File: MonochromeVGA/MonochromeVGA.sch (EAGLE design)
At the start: 12 parts

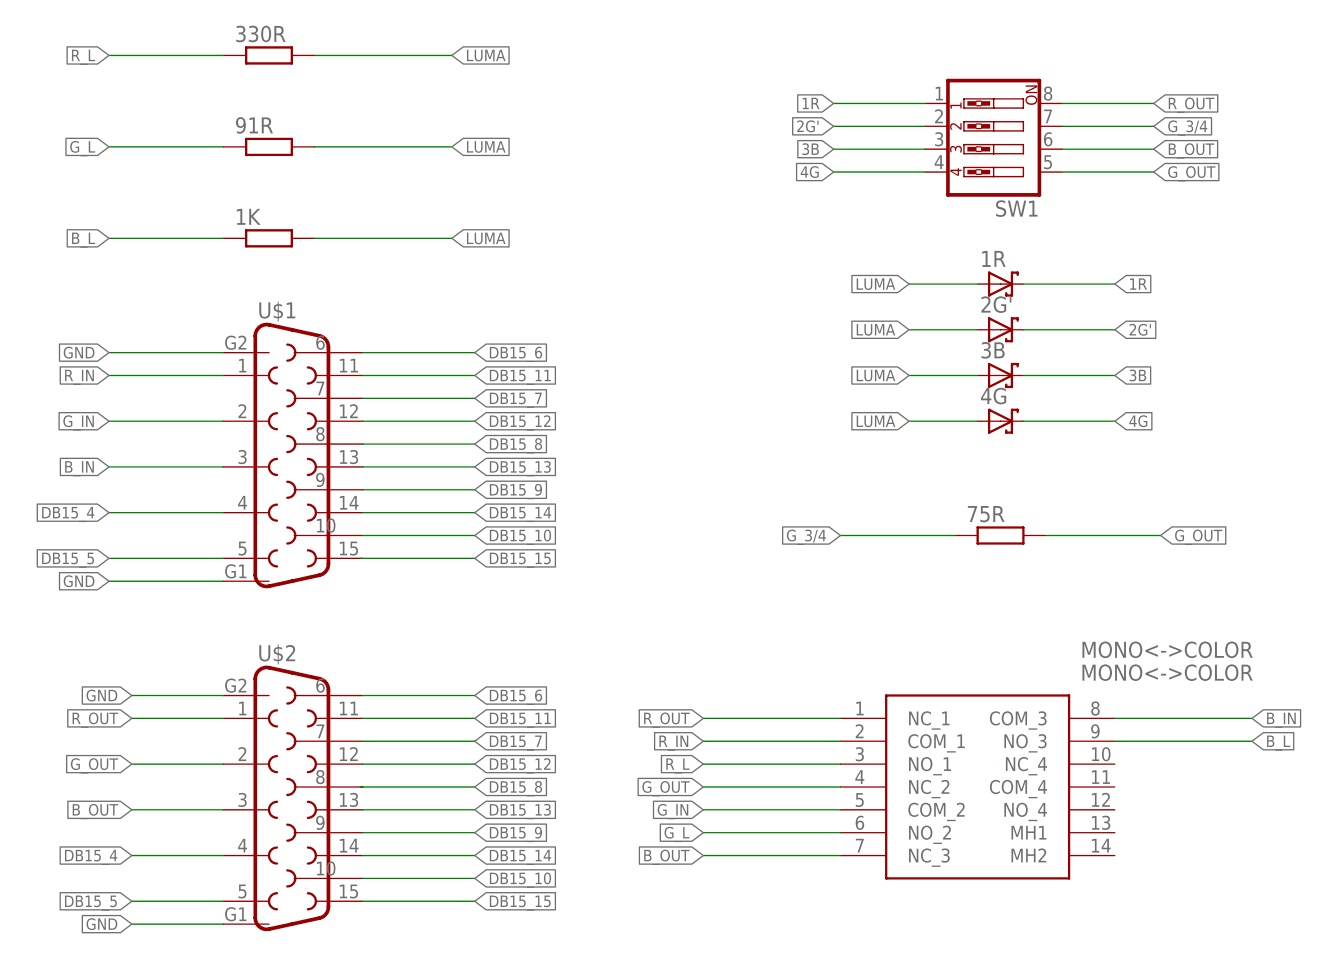
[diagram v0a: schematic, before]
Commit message: Add files via upload
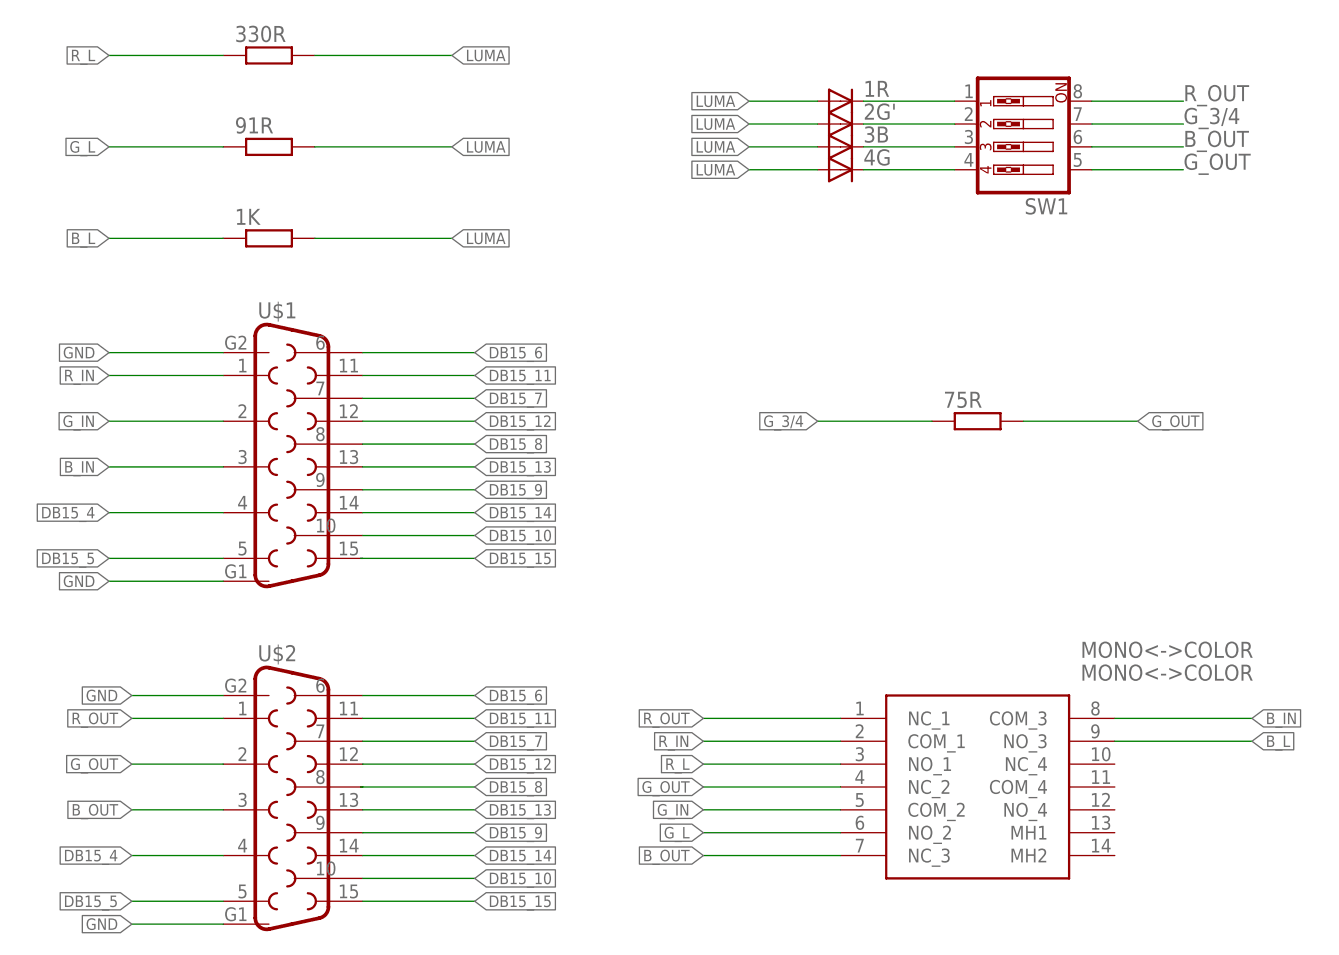
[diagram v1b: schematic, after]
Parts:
- 1R, 2G', 3B, 4G: device diode:SCHOTTKY-DIODEDO35-7 -> diode:DIODE-D-5
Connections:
- net 1R renamed N$6
- net 2G' renamed N$3
- net 3B renamed N$4
- net 4G renamed N$5
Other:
- moved on the sheet: 75R, SW1
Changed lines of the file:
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@@
 <part name="75R" library="resistor" deviceset="R-EU_" device="0204/5"/>
 <part name="MONO&lt;-&gt;COLOR" library="EG4208A" deviceset="EG4208A" device="" value="MONO&lt;-&gt;COLOR"/>
-<part name="2G'" library="diode" deviceset="SCHOTTKY-DIODE" device="DO35-7"/>
-<part name="3B" library="diode" deviceset="SCHOTTKY-DIODE" device="DO35-7"/>
-<part name="4G" library="diode" deviceset="SCHOTTKY-DIODE" device="DO35-7"/>
-<part name="1R" library="diode" deviceset="SCHOTTKY-DIODE" device="DO35-7"/>
+<part name="2G'" library="diode" deviceset="DIODE-" device="D-5"/>
+<part name="3B" library="diode" deviceset="DIODE-" device="D-5"/>
+<part name="4G" library="diode" deviceset="DIODE-" device="D-5"/>
+<part name="1R" library="diode" deviceset="DIODE-" device="D-5"/>
 </parts>
 <sheets>
@@
 </plain>
 <instances>
-<instance part="SW1" gate="A" x="93.218" y="86.106" rot="R180"/>
+<instance part="SW1" gate="A" x="96.52" y="86.36" rot="R180"/>
 <instance part="U$1" gate="G$1" x="15.24" y="53.34"/>
 <instance part="U$2" gate="G$1" x="15.24" y="15.24"/>
@@
 <instance part="91R" gate="G$1" x="12.7" y="86.36"/>
 <instance part="1K" gate="G$1" x="12.7" y="76.2"/>
-<instance part="75R" gate="G$1" x="93.98" y="43.18"/>
+<instance part="75R" gate="G$1" x="91.44" y="55.88"/>
 <instance part="MONO&lt;-&gt;COLOR" gate="G$1" x="76.2" y="22.86"/>
-<instance part="2G'" gate="G$1" x="93.98" y="66.04"/>
-<instance part="3B" gate="G$1" x="93.98" y="60.96"/>
-<instance part="4G" gate="G$1" x="93.98" y="55.88"/>
-<instance part="1R" gate="G$1" x="93.98" y="71.12"/>
+<instance part="2G'" gate="G$1" x="76.2" y="88.9"/>
+<instance part="3B" gate="G$1" x="76.2" y="86.36"/>
+<instance part="4G" gate="G$1" x="76.2" y="83.82"/>
+<instance part="1R" gate="G$1" x="76.2" y="91.44"/>
 </instances>
 <busses>
@@
 <segment>
 <pinref part="2G'" gate="G$1" pin="A"/>
-<wire x1="91.44" y1="66.04" x2="83.82" y2="66.04" width="0.1524" layer="91"/>
-<label x="83.82" y="66.04" size="1.27" layer="95" rot="R180" xref="yes"/>
+<wire x1="73.66" y1="88.9" x2="66.04" y2="88.9" width="0.1524" layer="91"/>
+<label x="66.04" y="88.9" size="1.27" layer="95" rot="R180" xref="yes"/>
 </segment>
 <segment>
 <pinref part="3B" gate="G$1" pin="A"/>
-<wire x1="91.44" y1="60.96" x2="83.82" y2="60.96" width="0.1524" layer="91"/>
-<label x="83.82" y="60.96" size="1.27" layer="95" rot="R180" xref="yes"/>
+<wire x1="73.66" y1="86.36" x2="66.04" y2="86.36" width="0.1524" layer="91"/>
+<label x="66.04" y="86.36" size="1.27" layer="95" rot="R180" xref="yes"/>
 </segment>
 <segment>
 <pinref part="4G" gate="G$1" pin="A"/>
-<wire x1="91.44" y1="55.88" x2="83.82" y2="55.88" width="0.1524" layer="91"/>
-<label x="83.82" y="55.88" size="1.27" layer="95" rot="R180" xref="yes"/>
+<wire x1="73.66" y1="83.82" x2="66.04" y2="83.82" width="0.1524" layer="91"/>
+<label x="66.04" y="83.82" size="1.27" layer="95" rot="R180" xref="yes"/>
 </segment>
 <segment>
 <pinref part="1R" gate="G$1" pin="A"/>
-<wire x1="91.44" y1="71.12" x2="83.82" y2="71.12" width="0.1524" layer="91"/>
-<label x="83.82" y="71.12" size="1.27" layer="95" rot="R180" xref="yes"/>
+<wire x1="73.66" y1="91.44" x2="66.04" y2="91.44" width="0.1524" layer="91"/>
+<label x="66.04" y="91.44" size="1.27" layer="95" rot="R180" xref="yes"/>
 </segment>
 </net>
@@
 <segment>
 <pinref part="SW1" gate="A" pin="8"/>
-<wire x1="100.838" y1="91.186" x2="110.998" y2="91.186" width="0.1524" layer="91"/>
-<label x="110.998" y="91.186" size="1.27" layer="95" xref="yes"/>
+<wire x1="104.14" y1="91.44" x2="114.3" y2="91.44" width="0.1524" layer="91"/>
+<label x="114.3" y="91.44" size="1.778" layer="95"/>
 </segment>
 <segment>
@@
 <segment>
 <pinref part="SW1" gate="A" pin="5"/>
-<wire x1="100.838" y1="83.566" x2="110.998" y2="83.566" width="0.1524" layer="91"/>
-<label x="110.998" y="83.566" size="1.27" layer="95" xref="yes"/>
+<wire x1="104.14" y1="83.82" x2="114.3" y2="83.82" width="0.1524" layer="91"/>
+<label x="114.3" y="83.82" size="1.778" layer="95"/>
 </segment>
 <segment>
@@
 <segment>
 <pinref part="75R" gate="G$1" pin="2"/>
-<wire x1="99.06" y1="43.18" x2="111.76" y2="43.18" width="0.1524" layer="91"/>
-<label x="111.76" y="43.18" size="1.27" layer="95" xref="yes"/>
+<wire x1="96.52" y1="55.88" x2="109.22" y2="55.88" width="0.1524" layer="91"/>
+<label x="109.22" y="55.88" size="1.27" layer="95" xref="yes"/>
 </segment>
 </net>
@@
 <segment>
 <pinref part="SW1" gate="A" pin="6"/>
-<wire x1="100.838" y1="86.106" x2="110.998" y2="86.106" width="0.1524" layer="91"/>
-<label x="110.998" y="86.106" size="1.27" layer="95" xref="yes"/>
+<wire x1="104.14" y1="86.36" x2="114.3" y2="86.36" width="0.1524" layer="91"/>
+<label x="114.3" y="86.36" size="1.778" layer="95"/>
 </segment>
 <segment>
@@
 <segment>
 <pinref part="SW1" gate="A" pin="7"/>
-<wire x1="100.838" y1="88.646" x2="110.998" y2="88.646" width="0.1524" layer="91"/>
-<label x="110.998" y="88.646" size="1.27" layer="95" xref="yes"/>
+<wire x1="104.14" y1="88.9" x2="114.3" y2="88.9" width="0.1524" layer="91"/>
+<label x="114.3" y="88.9" size="1.778" layer="95"/>
 </segment>
 <segment>
 <pinref part="75R" gate="G$1" pin="1"/>
-<wire x1="88.9" y1="43.18" x2="76.2" y2="43.18" width="0.1524" layer="91"/>
-<label x="76.2" y="43.18" size="1.27" layer="95" rot="R180" xref="yes"/>
+<wire x1="86.36" y1="55.88" x2="73.66" y2="55.88" width="0.1524" layer="91"/>
+<label x="73.66" y="55.88" size="1.27" layer="95" rot="R180" xref="yes"/>
 </segment>
 </net>
@@
 </segment>
 </net>
-<net name="1R" class="0">
+<net name="N$3" class="0">
+<segment>
+<pinref part="2G'" gate="G$1" pin="C"/>
+<pinref part="SW1" gate="A" pin="2"/>
+<wire x1="78.74" y1="88.9" x2="88.9" y2="88.9" width="0.1524" layer="91"/>
+</segment>
+</net>
+<net name="N$4" class="0">
+<segment>
+<pinref part="3B" gate="G$1" pin="C"/>
+<pinref part="SW1" gate="A" pin="3"/>
+<wire x1="78.74" y1="86.36" x2="88.9" y2="86.36" width="0.1524" layer="91"/>
+</segment>
+</net>
+<net name="N$5" class="0">
+<segment>
+<pinref part="4G" gate="G$1" pin="C"/>
+<pinref part="SW1" gate="A" pin="4"/>
+<wire x1="78.74" y1="83.82" x2="88.9" y2="83.82" width="0.1524" layer="91"/>
+</segment>
+</net>
+<net name="N$6" class="0">
 <segment>
 <pinref part="1R" gate="G$1" pin="C"/>
-<wire x1="96.52" y1="71.12" x2="106.68" y2="71.12" width="0.1524" layer="91"/>
-<label x="106.68" y="71.12" size="1.27" layer="95" xref="yes"/>
-</segment>
-<segment>
 <pinref part="SW1" gate="A" pin="1"/>
-<wire x1="85.598" y1="91.186" x2="75.438" y2="91.186" width="0.1524" layer="91"/>
-<label x="75.438" y="91.186" size="1.27" layer="95" rot="R180" xref="yes"/>
-</segment>
-</net>
-<net name="2G'" class="0">
-<segment>
-<pinref part="2G'" gate="G$1" pin="C"/>
-<wire x1="96.52" y1="66.04" x2="106.68" y2="66.04" width="0.1524" layer="91"/>
-<label x="106.68" y="66.04" size="1.27" layer="95" xref="yes"/>
-</segment>
-<segment>
-<pinref part="SW1" gate="A" pin="2"/>
-<wire x1="85.598" y1="88.646" x2="75.438" y2="88.646" width="0.1524" layer="91"/>
-<label x="75.438" y="88.646" size="1.27" layer="95" rot="R180" xref="yes"/>
-</segment>
-</net>
-<net name="3B" class="0">
-<segment>
-<pinref part="3B" gate="G$1" pin="C"/>
-<wire x1="96.52" y1="60.96" x2="106.68" y2="60.96" width="0.1524" layer="91"/>
-<label x="106.68" y="60.96" size="1.27" layer="95" xref="yes"/>
-</segment>
-<segment>
-<pinref part="SW1" gate="A" pin="3"/>
-<wire x1="85.598" y1="86.106" x2="75.438" y2="86.106" width="0.1524" layer="91"/>
-<label x="75.438" y="86.106" size="1.27" layer="95" rot="R180" xref="yes"/>
-</segment>
-</net>
-<net name="4G" class="0">
-<segment>
-<pinref part="4G" gate="G$1" pin="C"/>
-<wire x1="96.52" y1="55.88" x2="106.68" y2="55.88" width="0.1524" layer="91"/>
-<label x="106.68" y="55.88" size="1.27" layer="95" xref="yes"/>
-</segment>
-<segment>
-<pinref part="SW1" gate="A" pin="4"/>
-<wire x1="85.598" y1="83.566" x2="75.438" y2="83.566" width="0.1524" layer="91"/>
-<label x="75.438" y="83.566" size="1.27" layer="95" rot="R180" xref="yes"/>
-</segment>
-</net>
+<wire x1="78.74" y1="91.44" x2="88.9" y2="91.44" width="0.1524" layer="91"/>
+</segment>
+</net>
